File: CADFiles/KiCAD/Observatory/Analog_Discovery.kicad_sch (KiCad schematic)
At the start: 1 part, among them J2 Analog Discovery Connection

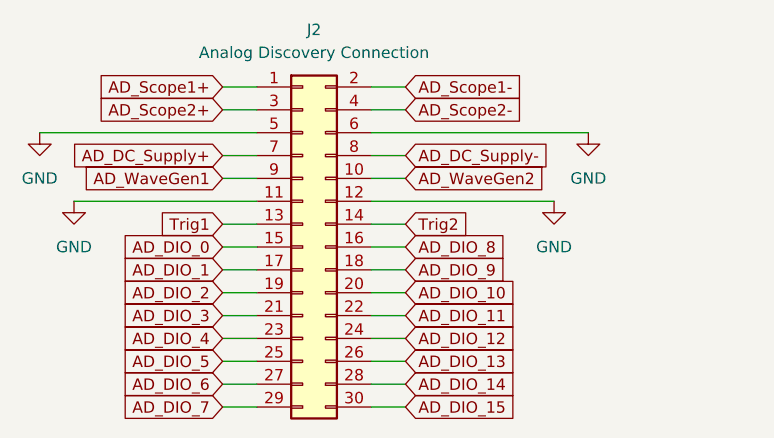
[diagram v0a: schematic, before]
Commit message: Begin REV 2
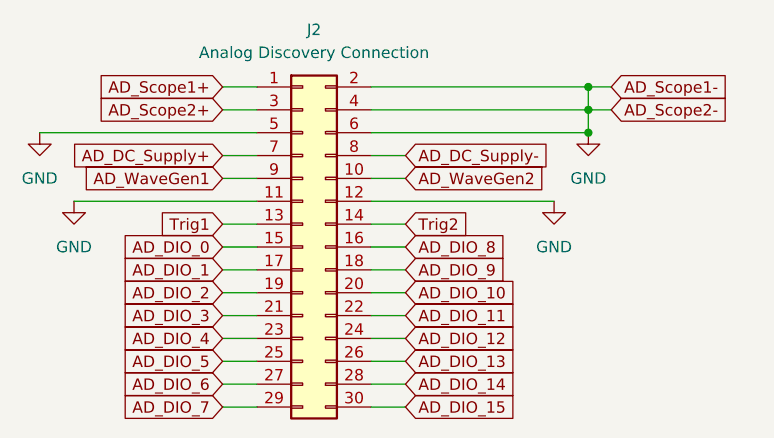
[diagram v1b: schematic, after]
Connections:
- net AD_Scope1- is gone; now on net GND: J2.2 (Pin_2)
- net AD_Scope2- is gone; now on net GND: J2.4 (Pin_4)
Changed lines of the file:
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@@
 (kicad_sch
-	(version 20231120)
+	(version 20250114)
 	(generator "eeschema")
-	(generator_version "8.0")
+	(generator_version "9.0")
 	(paper "A4")
+	(junction
+		(at 158.75 81.28)
+		(diameter 0)
+		(color 0 0 0 0)
+	)
+	(junction
+		(at 158.75 86.36)
+		(diameter 0)
+		(color 0 0 0 0)
+	)
+	(junction
+		(at 158.75 83.82)
+		(diameter 0)
+		(color 0 0 0 0)
+	)
 	(wire
 		(pts
-			(xy 134.62 81.28) (xy 138.43 81.28)
+			(xy 134.62 81.28) (xy 158.75 81.28)
 		)
 		(stroke
@@
 	(wire
 		(pts
+			(xy 158.75 81.28) (xy 161.29 81.28)
+		)
+		(stroke
+			(width 0)
+			(type default)
+		)
+	)
+	(wire
+		(pts
 			(xy 134.62 116.84) (xy 138.43 116.84)
 		)
@@
 	(wire
 		(pts
+			(xy 158.75 81.28) (xy 158.75 83.82)
+		)
+		(stroke
+			(width 0)
+			(type default)
+		)
+	)
+	(wire
+		(pts
 			(xy 134.62 88.9) (xy 138.43 88.9)
 		)
@@
 	(wire
 		(pts
+			(xy 158.75 83.82) (xy 161.29 83.82)
+		)
+		(stroke
+			(width 0)
+			(type default)
+		)
+	)
+	(wire
+		(pts
 			(xy 134.62 106.68) (xy 138.43 106.68)
 		)
@@
 	(wire
 		(pts
+			(xy 158.75 83.82) (xy 158.75 86.36)
+		)
+		(stroke
+			(width 0)
+			(type default)
+		)
+	)
+	(wire
+		(pts
 			(xy 134.62 93.98) (xy 154.94 93.98)
 		)
@@
 	(wire
 		(pts
-			(xy 134.62 83.82) (xy 138.43 83.82)
+			(xy 134.62 83.82) (xy 158.75 83.82)
 		)
 		(stroke
@@
 			"uAMAAAAAwEC4AwAAAADAQLgDAAAAAMBAuAMAAAAAwEC4AwAAAADAQLgDAAAAAMBAuAMAAAAAwEC4"
 			"AwAAAADAQLgDAAAAAMBAuAMAAAAAwEC4AwAAAADAQLgDAAAAAMBAuAMAAAAAwEC4AwAAAADAQLgD"
-			"AAAAAMAgjLOiEIv63qMAAAAASUVORK5CYII="
+			"AAAAAMAgjLOiEIv63qMAAAAASUVORK5CYIIAZAAAADEAAAAxAAAAYQAAAGQAAABsAAAAOQAAAFoA"
+			"AABVAAAAMgAAADEAAABPAAAAaAAAAFgAAABrAAAAcgAAAHcAAABPAAAARAAAADQAAABpAAAASwAA"
+			"ACsAAAB1AAAAYwAAAGEAAABqAAAAMAAAAEwAAAAwAAAAZAAAADIAAABJAAAANAAAAFoAAABZAAAA"
+			"YgAAAHkAAABQAAAAcAAAAFAAAABiAAAAawAAADAAAABtAAAAWAAAAGoAAAA2AAAAbwAAAHQAAABT"
+			"AAAAWQAAAFYAAAArAAAAeQAAAEYAAABWAAAAWQAAAHUAAABOAAAAYgAAADgAAABPAAAAOAAAAFgA"
+			"AABWAAAAQgAAADkAAAB0AAAAKwAAAGEAAAAwAAAAdAAAADkAAABkAAAAeAAAAFoAAABqAAAAdAAA"
+			"ADIAAAA2AAAAOQAAAG0AAABUAAAANQAAAG4AAAAvAAAAMwAAAGUAAABtAAAAYgAAACsAAABwAAAA"
+			"eAAAAFUAAAB0AAAATAAAAHUAAAA0AAAAZQAAAHcAAABXAAAAWAAAAEIAAAB5AAAAUwAAAFIAAAB4"
+			"AAAAYgAAAEgAAAB0AAAAQQAAAGMAAABZAAAAegAAADMAAABuAAAAWQAAAFUAAABWAAAAOQAAAHIA"
+			"AABSAAAAaQAAAFUAAABrAAAAaAAAAFcAAABSAAAATgAAAEMAAABMAAAASQAAAGkAAABnAAAAWQAA"
+			"AFEAAABlAAAASQAAAEwAAABmAAAAOQAAADMAAABlAAAARgAAAGQAAABSAAAAawAAAGEAAABaAAAA"
+			"TgAAAEsAAAArAAAAUwAAAGEAAABaAAAAWgAAAHcAAABnAAAAaAAAAGgAAABCAAAAQgAAAEMAAABD"
+			"AAAAQwAAAEgAAABFAAAAQgAAAEEAAAByAAAAdQAAAHMAAAB4AAAAdgAAAHMAAABEAAAAegAAAFcA"
+			"AAA1AAAAQwAAAEEAAAA3AAAATAAAAEsAAABoAAAAOAAAAHkAAAA0AAAATgAAAGMAAABUAAAARQAA"
+			"AFUAAABHAAAAcQAAAHQAAABxAAAAdgAAAE0AAABqAAAAaAAAADIAAAA3AAAATwAAADAAAABWAAAA"
+			"RwAAAFUAAABKAAAAdAAAAFQAAABrAAAAYwAAAFQAAAAxAAAAOQAAAEIAAAB5AAAAeAAAAHEAAABm"
+			"AAAAMgAAAE4AAAB0AAAAUAAAAGQAAABLAAAAWQAAAGYAAAB6AAAAUgAAADIAAAAxAAAAOAAAADYA"
+			"AABFAAAAcQAAAHAAAABnAAAAdgAAAGQAAAByAAAAYwAAAHkAAAByAAAARwAAAGQAAAA3AAAAYgAA"
+			"AEMAAABrAAAATgAAAFAAAAA5AAAAMQAAAA=="
 		)
 	)
@@
 	(global_label "AD_Scope2-"
 		(shape input)
-		(at 138.43 83.82 0)
+		(at 161.29 83.82 0)
 		(fields_autoplaced yes)
 		(effects
@@
 		)
 		(property "Intersheetrefs" "${INTERSHEET_REFS}"
-			(at 153.208 83.82 0)
+			(at 176.068 83.82 0)
 			(effects
 				(font
@@
 	(global_label "AD_Scope1-"
 		(shape input)
-		(at 138.43 81.28 0)
+		(at 161.29 81.28 0)
 		(fields_autoplaced yes)
 		(effects
@@
 		)
 		(property "Intersheetrefs" "${INTERSHEET_REFS}"
-			(at 153.208 81.28 0)
+			(at 176.068 81.28 0)
 			(effects
 				(font
